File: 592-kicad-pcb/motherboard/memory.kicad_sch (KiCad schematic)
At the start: 21 parts, among them J19 Micro_SD_Card, J20 Conn_02x01, U13 W25Q32JVSS, U14 SN74LVC1G3157DBVR

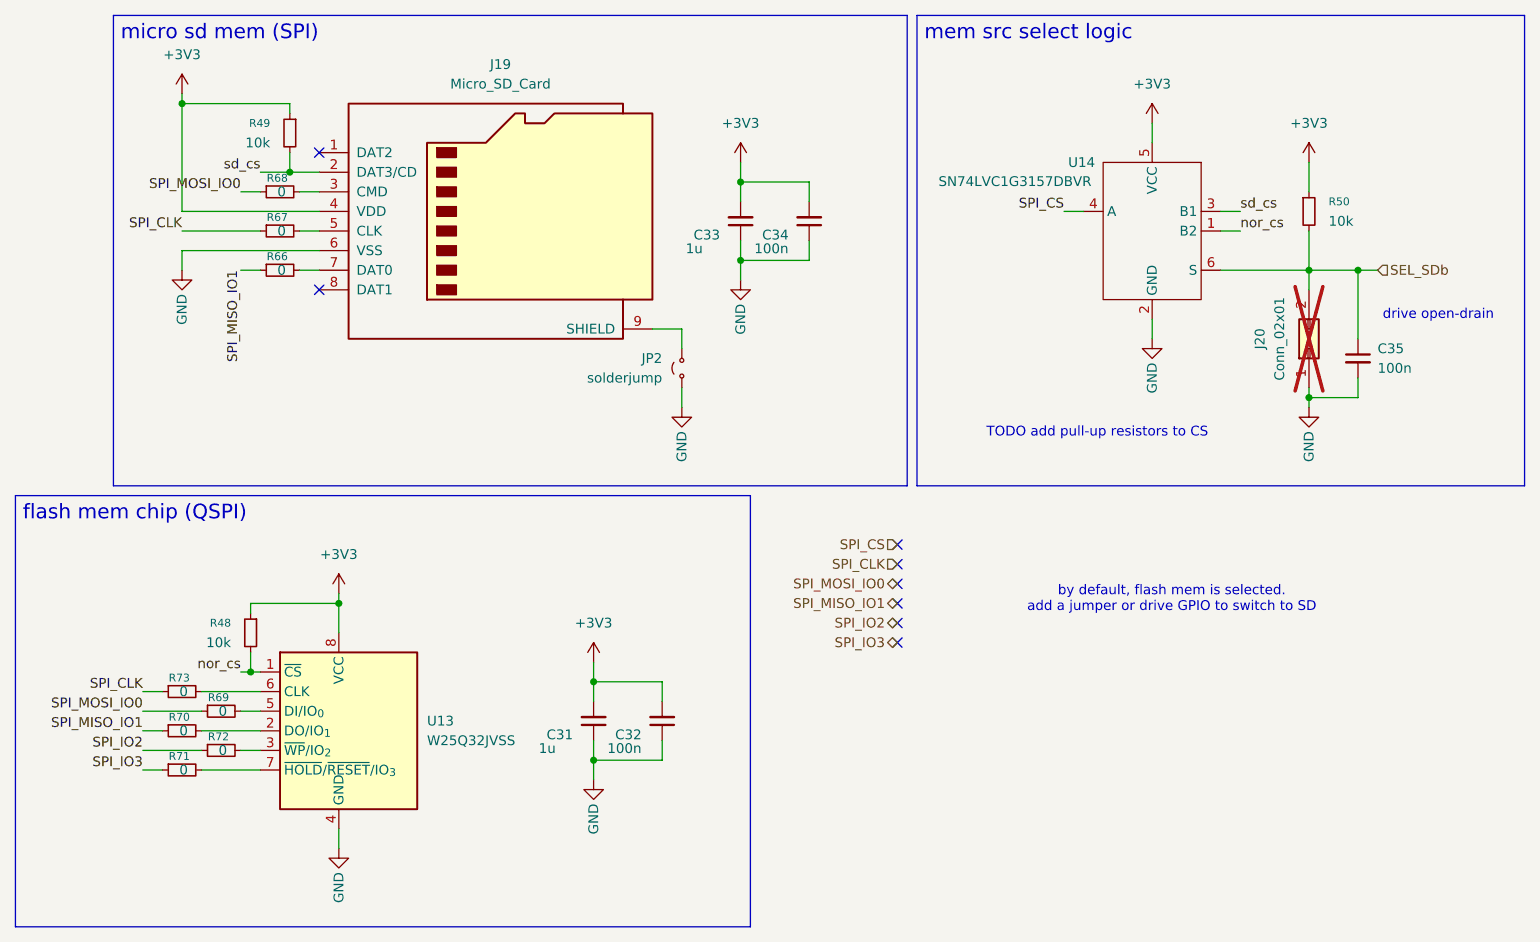
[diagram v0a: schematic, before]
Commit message: finalize termination
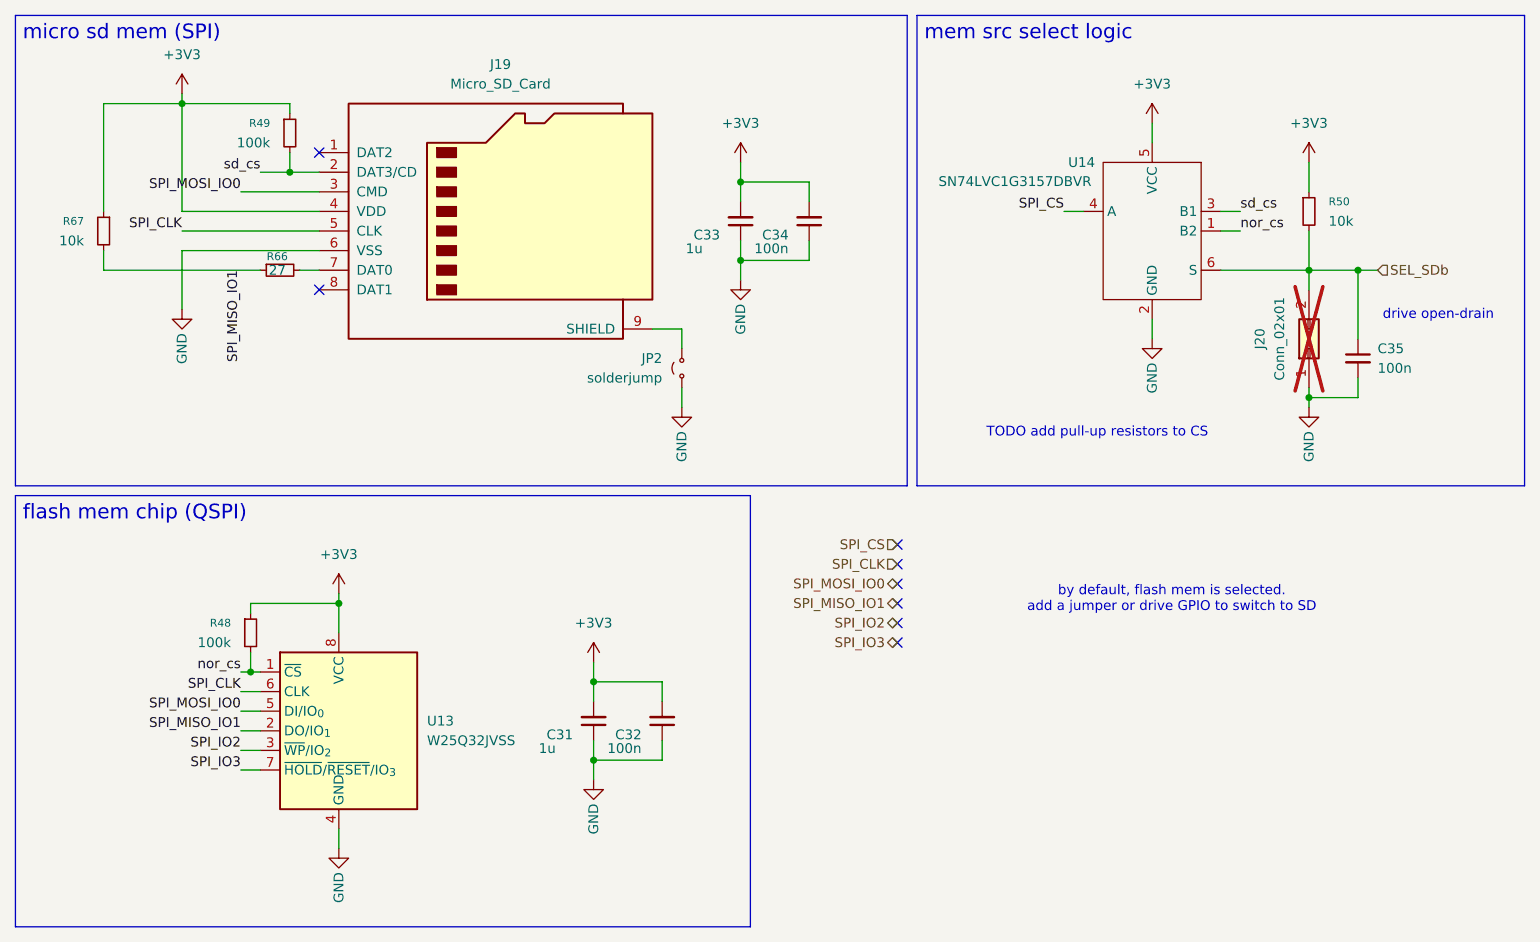
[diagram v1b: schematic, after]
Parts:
- removed R68, R69, R70, R71, R72, R73: 0, Resistor_SMD:R_0402_1005Metric, symbol Device:R_Small
- R48, R49: value 10k -> 100k; footprint Resistor_SMD:R_0402_1005Metric -> (none); LCSC C25744 -> (none)
- R66: value 0 -> 27
- R67: value 0 -> 10k; LCSC (none) -> C25744
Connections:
- net +3V3: now also R67.1
- net SPI_CLK: now also J19.5 (CLK), U13.6 (CLK); no longer R67.1
- net SPI_IO2: now also U13.3 (~{WP}/IO_{2})
- net SPI_IO3: now also U13.7 (~{HOLD}/~{RESET}/IO_{3})
- net SPI_MISO_IO1: now also R67.2, U13.2 (DO/IO_{1})
- net SPI_MOSI_IO0: now also J19.3 (CMD), U13.5 (DI/IO_{0})
